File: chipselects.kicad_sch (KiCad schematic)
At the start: 12 parts, among them J1 VERA, K2 VERA INTERRUPT SELECT, K3 AUDIO OUT, SW1 VERA ADDR, SW2 Keyboard/Printer, U18 74LS688, U19 74LS688, U20 74LS138, U21 74LS138

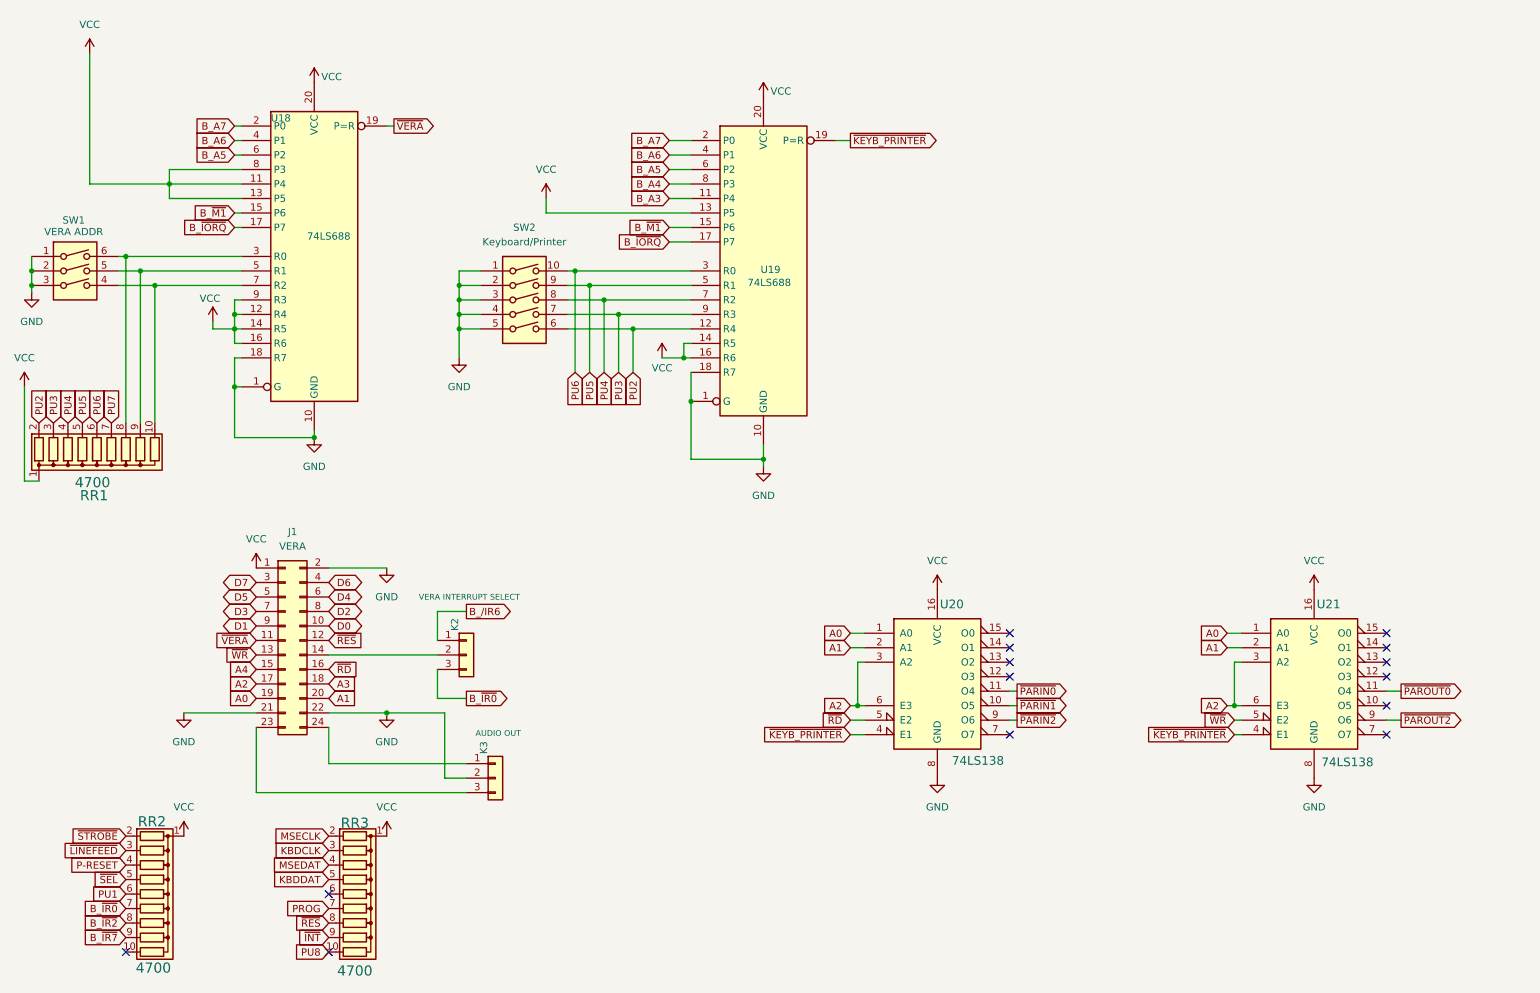
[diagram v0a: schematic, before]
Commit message: V1.1
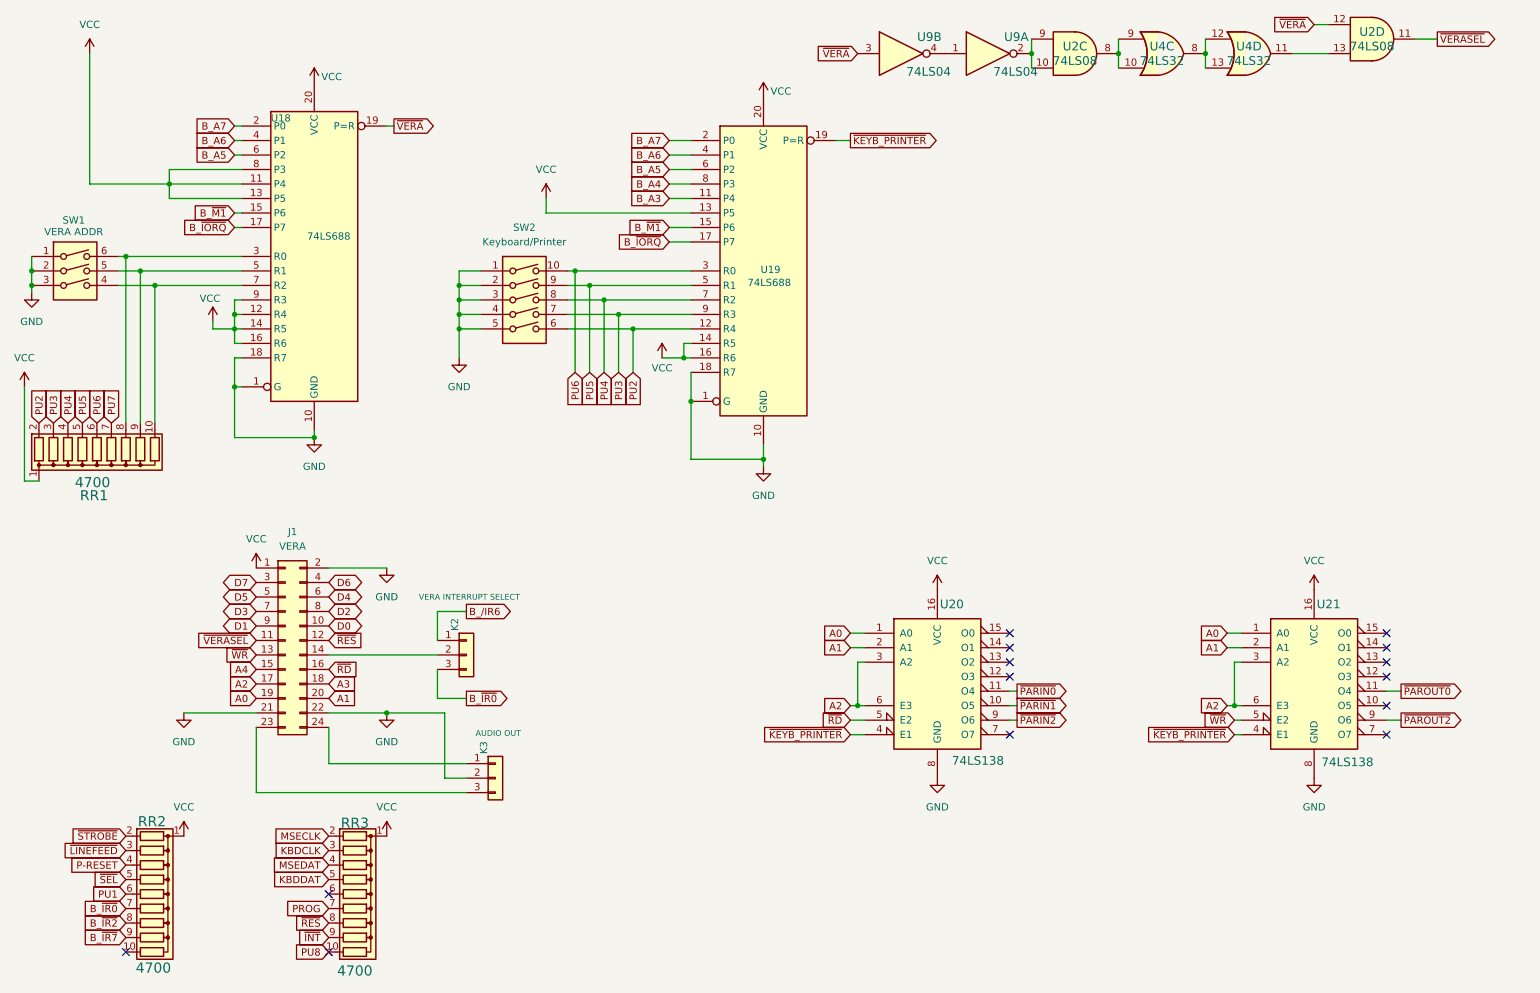
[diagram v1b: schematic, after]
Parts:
- added U2: 74LS08, Custom:STD_DDW_DIP14, symbol 74xx:74LS08
- added U4: 74LS32, Custom:STD_DDW_DIP14, symbol 74xx:74LS32
- added U9: 74LS04, Custom:STD_DDW_DIP14, symbol 74xx:74LS04
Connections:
- net ~{VERA}: now also U2.12, U9.3; no longer J1.11 (Pin_11)
- new net: U2.8, U4.10, U4.9
- new net: U4.12, U4.13, U4.8
- new net: U2.10, U2.9, U9.2
- new net: U2.13, U4.11
- new net: U9.1, U9.4
- new net ~{VERASEL}: J1.11 (Pin_11), U2.11
